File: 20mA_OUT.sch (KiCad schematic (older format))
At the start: 7 parts, among them Q1 IRF540N, U4 LM321

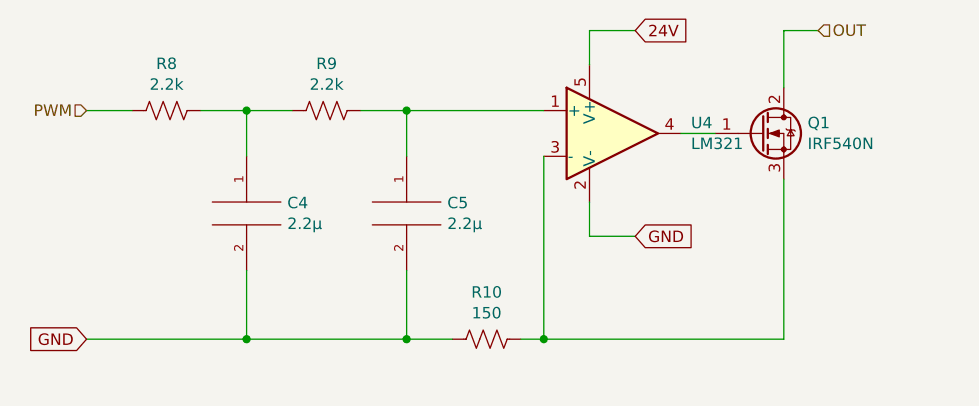
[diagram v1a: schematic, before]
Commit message: Comments and Notation for clarity
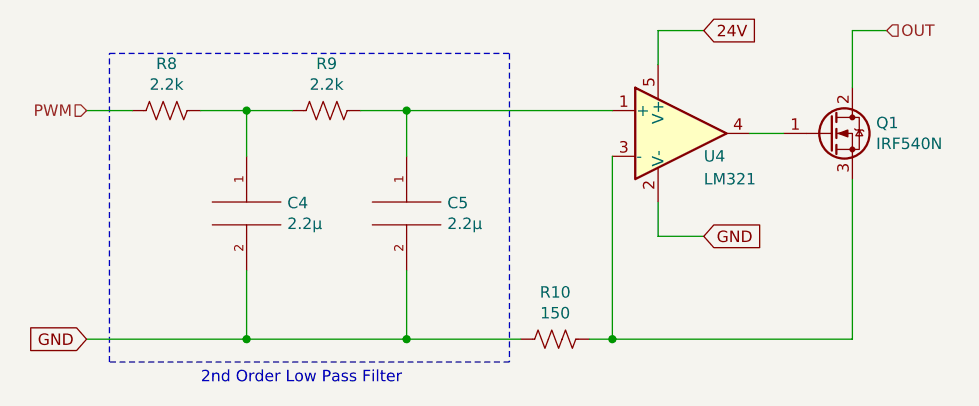
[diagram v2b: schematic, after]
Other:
- note added: "2nd Order Low Pass Filter"
- moved on the sheet: Q1, R10, U4
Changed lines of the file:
@@
 encoding utf-8
 Sheet 3 6
-Title ""
-Date ""
-Rev ""
-Comp ""
-Comment1 ""
+Title "PWM to 20mA Output"
+Date "2021-05-25"
+Rev "1"
+Comp "Harsch Systems"
+Comment1 "Tyler Stowell"
 Comment2 ""
 Comment3 ""
@@
 L Amplifier_Operational:LM321 U?
 U 1 1 60ABF5F3
-P 6400 3700
+P 6700 3700
 AR Path="/60A68B69/60ABF5F3" Ref="U?"  Part="1"
 AR Path="/60ABD2CD/60ABF5F3" Ref="U4"  Part="1"
-F 0 "U4" H 6744 3746 50  0000 L CNN
-F 1 "LM321" H 6744 3655 50  0000 L CNN
-F 2 "Package_TO_SOT_SMD:SOT-23-5" H 6400 3700 50  0001 C CNN
-F 3 "http://www.ti.com/lit/ds/symlink/lm321.pdf" H 6400 3700 50  0001 C CNN
-	1    6400 3700
+F 0 "U4" H 6800 3600 50  0000 L CNN
+F 1 "LM321" H 6800 3500 50  0000 L CNN
+F 2 "Package_TO_SOT_SMD:SOT-23-5" H 6700 3700 50  0001 C CNN
+F 3 "http://www.ti.com/lit/ds/symlink/lm321.pdf" H 6700 3700 50  0001 C CNN
+	1    6700 3700
 	1    0    0    -1
 $EndComp
@@
 L Device:R_US R?
 U 1 1 60ABF5FF
-P 5850 4600
+P 6150 4600
 AR Path="/60A68B69/60ABF5FF" Ref="R?"  Part="1"
 AR Path="/60ABD2CD/60ABF5FF" Ref="R10"  Part="1"
-F 0 "R10" V 5645 4600 50  0000 C CNN
-F 1 "150" V 5736 4600 50  0000 C CNN
-F 2 "" V 5890 4590 50  0001 C CNN
-F 3 "~" H 5850 4600 50  0001 C CNN
-	1    5850 4600
+F 0 "R10" V 5945 4600 50  0000 C CNN
+F 1 "150" V 6036 4600 50  0000 C CNN
+F 2 "" V 6190 4590 50  0001 C CNN
+F 3 "~" H 6150 4600 50  0001 C CNN
+	1    6150 4600
 	0    1    1    0
 $EndComp
@@
 	5500 3600 5500 3800
 Wire Wire Line
-	5500 3600 6100 3600
-Connection ~ 5500 3600
+	6400 3800 6400 4600
 Wire Wire Line
-	6100 3800 6100 4600
-Wire Wire Line
-	6100 4600 6000 4600
-Wire Wire Line
-	5700 4600 5500 4600
+	6400 4600 6300 4600
 Wire Wire Line
 	4800 4300 4800 4600
@@
 Wire Wire Line
 	5500 4300 5500 4600
-Connection ~ 5500 4600
 Wire Wire Line
 	5500 4600 4800 4600
-Text HLabel 7300 3250 2    50   Input ~ 0
+Text HLabel 7600 3250 2    50   Input ~ 0
 OUT
-Text GLabel 6500 4150 2    50   Input ~ 0
+Text GLabel 6800 4150 2    50   Input ~ 0
 GND
 Wire Wire Line
-	6300 4000 6300 4150
+	6600 4000 6600 4150
 Wire Wire Line
-	6300 4150 6500 4150
-Text GLabel 6500 3250 2    50   Input ~ 0
+	6600 4150 6800 4150
+Text GLabel 6800 3250 2    50   Input ~ 0
 24V
 Wire Wire Line
-	6300 3400 6300 3250
+	6600 3400 6600 3250
 Wire Wire Line
-	6300 3250 6500 3250
+	6600 3250 6800 3250
 $Comp
 L Transistor_FET:IRF540N Q1
 U 1 1 60AC135E
-P 7050 3700
-F 0 "Q1" H 7254 3746 50  0000 L CNN
-F 1 "IRF540N" H 7254 3655 50  0000 L CNN
-F 2 "Package_TO_SOT_THT:TO-220-3_Vertical" H 7300 3625 50  0001 L CIN
-F 3 "http://www.irf.com/product-info/datasheets/data/irf540n.pdf" H 7050 3700 50  0001 L CNN
-	1    7050 3700
+P 7350 3700
+F 0 "Q1" H 7554 3746 50  0000 L CNN
+F 1 "IRF540N" H 7554 3655 50  0000 L CNN
+F 2 "Package_TO_SOT_THT:TO-220-3_Vertical" H 7600 3625 50  0001 L CIN
+F 3 "http://www.irf.com/product-info/datasheets/data/irf540n.pdf" H 7350 3700 50  0001 L CNN
+	1    7350 3700
 	1    0    0    -1
 $EndComp
 Wire Wire Line
-	6700 3700 6850 3700
+	7000 3700 7150 3700
 Wire Wire Line
-	6100 4600 7150 4600
+	6400 4600 7450 4600
 Wire Wire Line
-	7150 4600 7150 3900
-Connection ~ 6100 4600
+	7450 4600 7450 3900
+Connection ~ 6400 4600
 Wire Wire Line
-	7150 3500 7150 3250
+	7450 3500 7450 3250
 Wire Wire Line
-	7150 3250 7300 3250
+	7450 3250 7600 3250
+Wire Wire Line
+	6000 4600 5500 4600
+Connection ~ 5500 4600
+Wire Wire Line
+	6400 3600 5500 3600
+Connection ~ 5500 3600
+Text Notes 4600 4800 0    50   ~ 0
+2nd Order Low Pass Filter
+Wire Notes Line
+	4200 4700 4200 3350
+Wire Notes Line
+	5950 4700 4200 4700
+Wire Notes Line
+	5950 3350 5950 4700
+Wire Notes Line
+	4200 3350 5950 3350
 $EndSCHEMATC
